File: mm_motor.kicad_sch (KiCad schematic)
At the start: 1 part, among them M1 N20_encoder

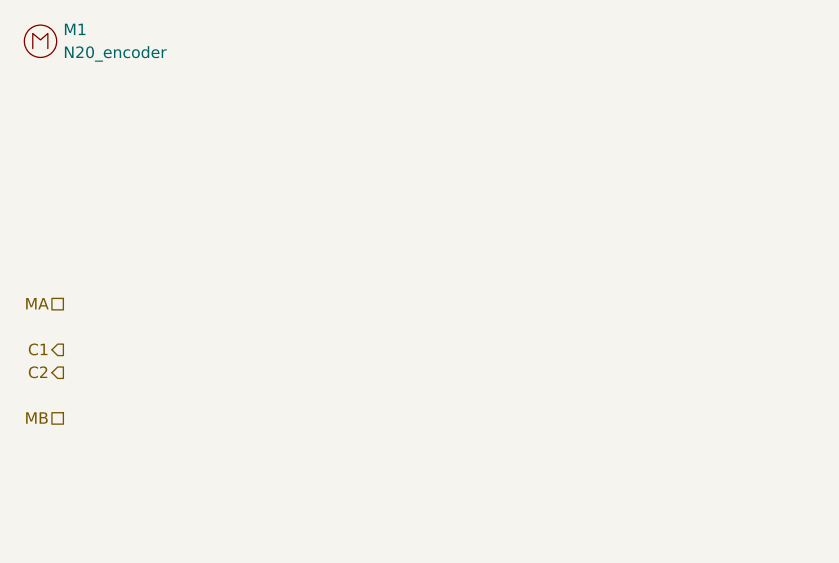
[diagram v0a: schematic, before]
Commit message: TP2
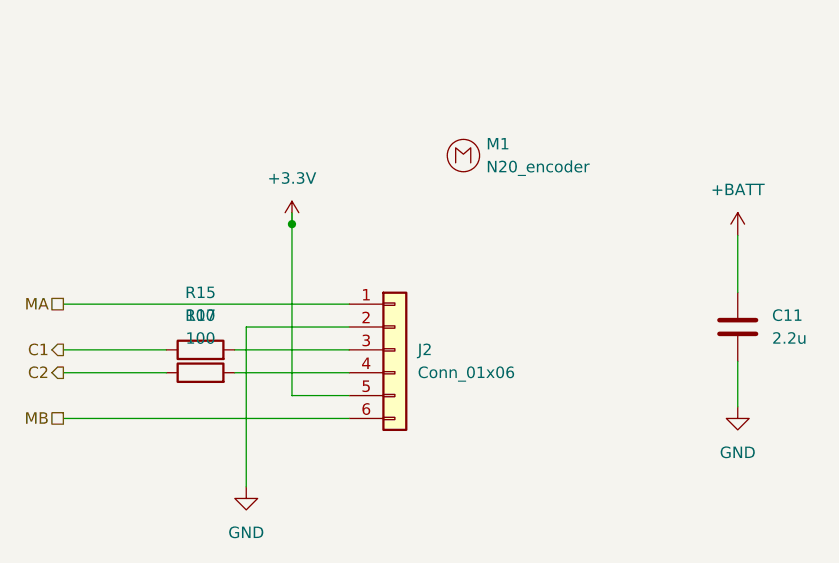
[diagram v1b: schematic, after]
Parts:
- added C11: 2.2u, Capacitor_SMD:C_0603_1608Metric, symbol Device:C
- added J2: Conn_01x06, Connector_PinHeader_2.54mm:PinHeader_1x06_P2.54mm_Vertical, symbol Connector_Generic:Conn_01x06
- added R15, R17: 100, Resistor_SMD:R_0603_1608Metric, symbol Device:R
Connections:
- net C1: now also R15.1
- net C2: now also R17.1
- net MA: now also J2.1 (Pin_1)
- net MB: now also J2.6 (Pin_6)
- new net: J2.3 (Pin_3), R15.2
- new net: J2.4 (Pin_4), R17.2
- new net +3.3V: J2.5 (Pin_5)
- new net +BATT: C11.1
- new net GND: C11.2, J2.2 (Pin_2)
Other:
- moved on the sheet: M1
